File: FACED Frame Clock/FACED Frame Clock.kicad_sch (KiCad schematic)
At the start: 49 parts, among them J1 Jack-DC, U1 LT1711xMS8, U2 LT1711xMS8, U3 LT1711xMS8, U4 LT1711xMS8, U5 Itsy_Bitsy_32u4, U6 SN74AC08PWR, U7 SN74AC08PWR

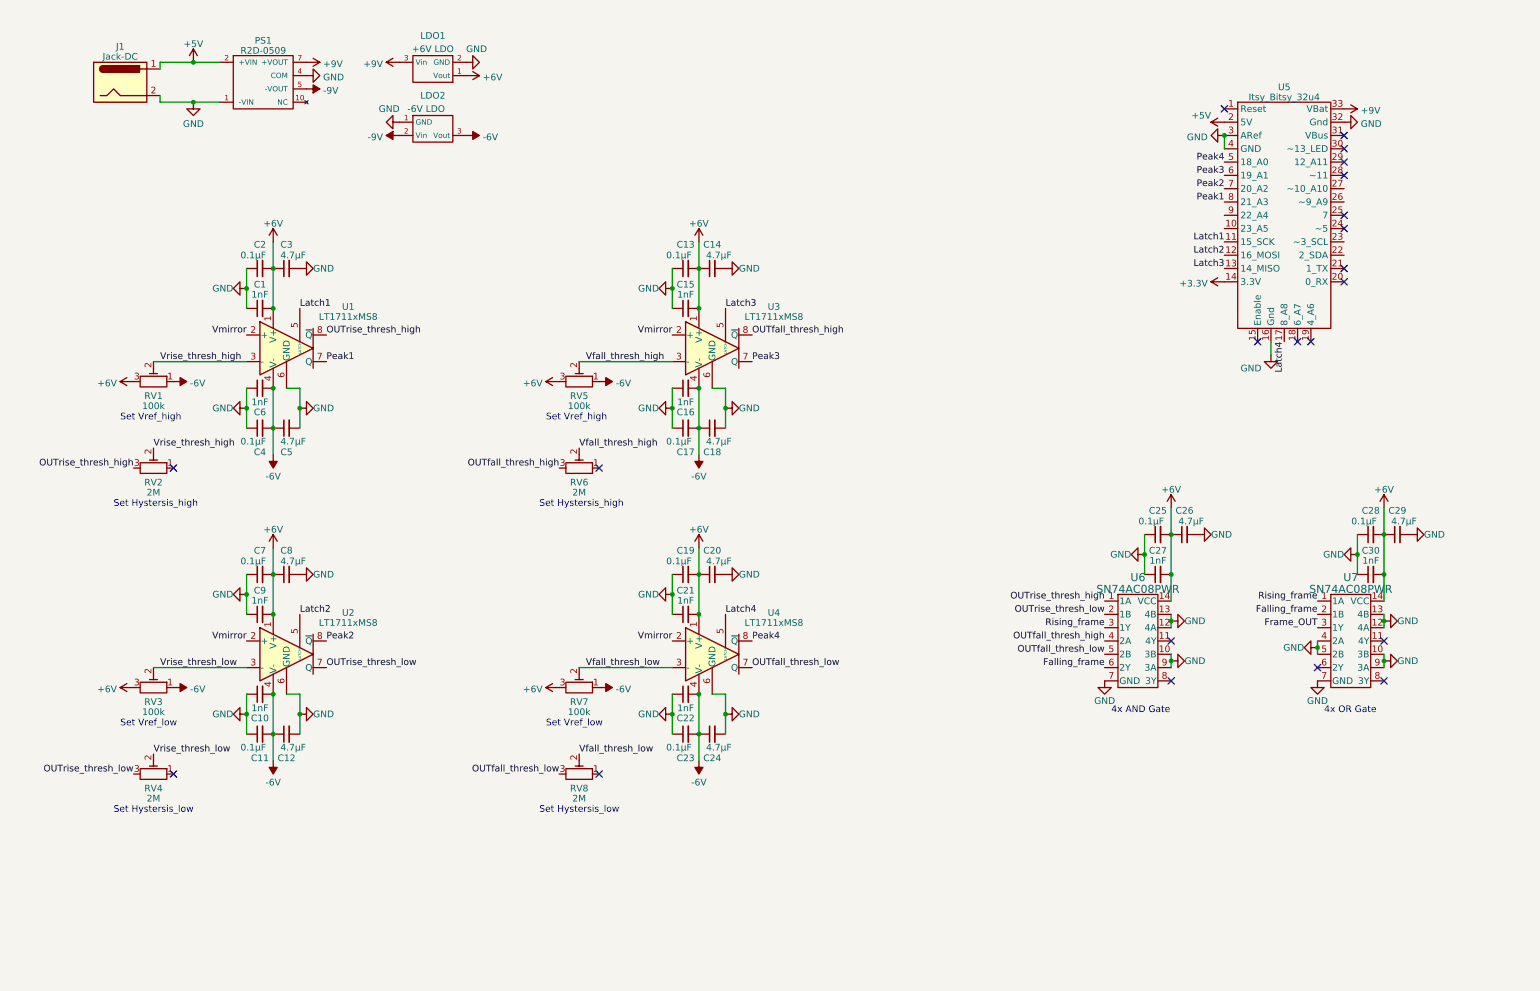
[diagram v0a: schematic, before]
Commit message: Label schematic
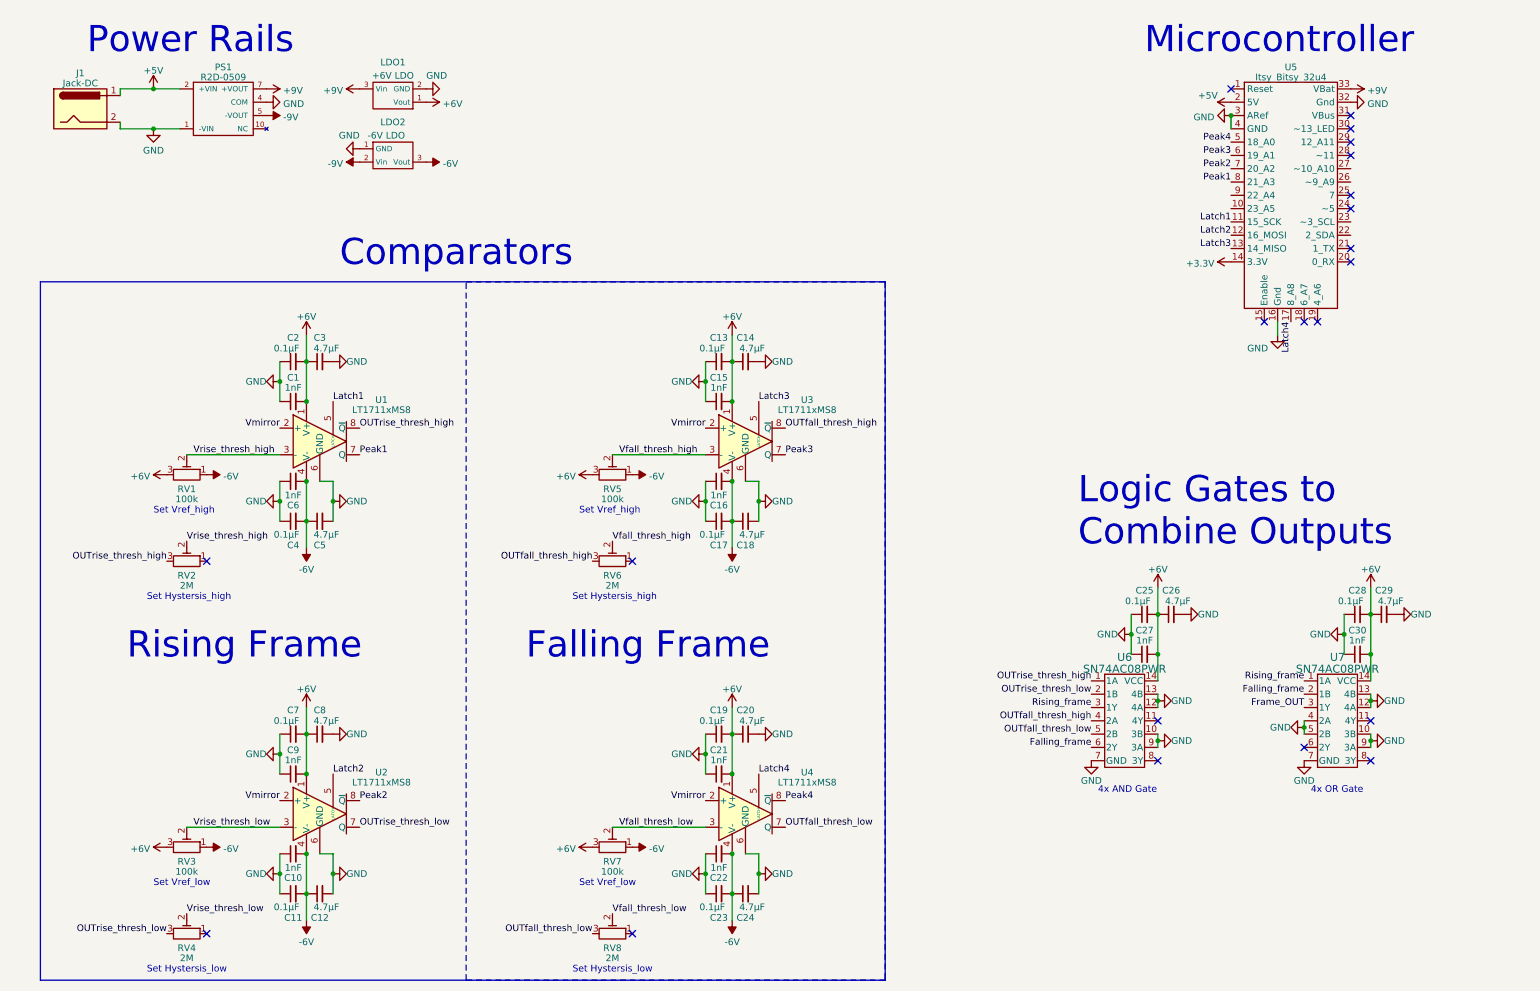
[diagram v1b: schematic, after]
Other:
- note added: "Comparators"
- note added: "Falling Frame"
- note added: "Logic Gates to Combine Outputs"
- note added: "Microcontroller"
- note added: "Power Rails"
- note added: "Rising Frame"
- moved on the sheet: C1, C10, C11, C12, C13, C14, C15, C16, C17, C18, C19, C2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

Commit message: Working draft of simplified version
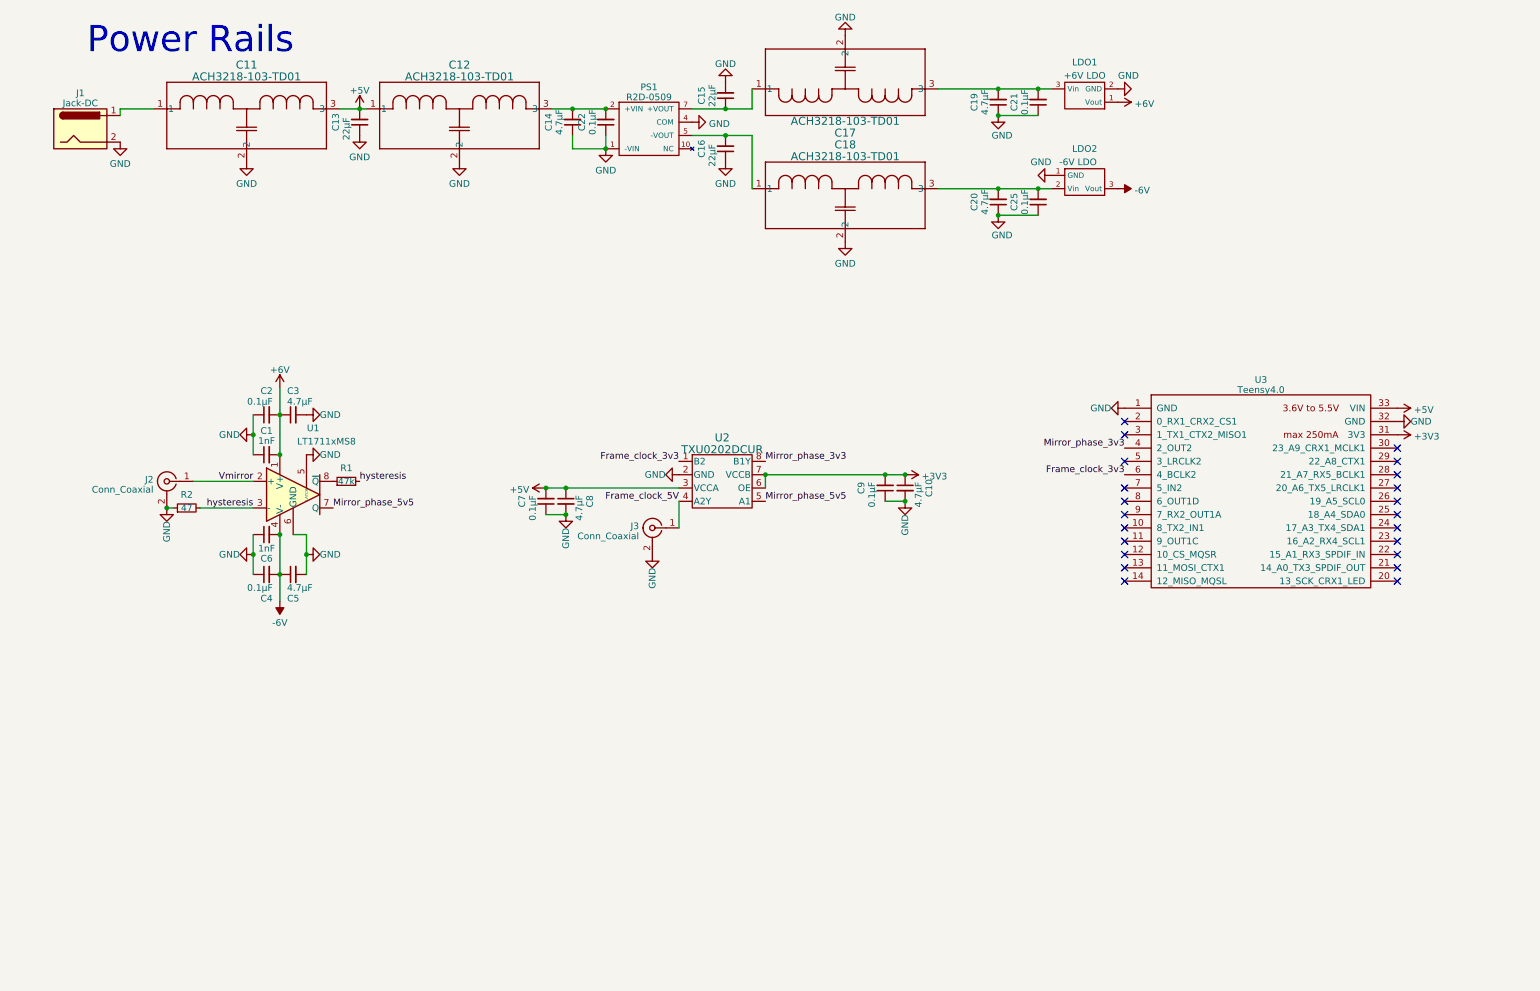
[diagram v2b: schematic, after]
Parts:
- removed C11, C17, C23, C28: 0.1µF, Capacitor_SMD:C_0603_1608Metric, symbol Device:C_Small
- removed C12, C18, C24, C26, C29: 4.7µF, Capacitor_SMD:C_0603_1608Metric, symbol Device:C_Small
- removed C27, C30: 1nF, Capacitor_SMD:C_0603_1608Metric, symbol Device:C_Small
- removed RV1, RV3, RV5, RV7: 100k, Custom footprints:TRIM_TS63Y104KT20, symbol Device:R_Potentiometer_Trim
- removed RV2, RV4, RV6, RV8: 2M, Custom footprints:TRIM_TS63Y104KT20, symbol Device:R_Potentiometer_Trim
- removed U2, U3, U4: LT1711xMS8, Package_SO:MSOP-8_3x3mm_P0.65mm, symbol Comparator:LT1711xMS8
- removed U5: Itsy_Bitsy_32u4, Custom footprints:Itsy Bitsy 32u4, symbol custom:Itsy_Bitsy_32u4
- removed U6, U7: SN74AC08PWR, PW14, symbol Custom:SN74AC08PWR
- added C11: ACH3218-103-TD01, Custom footprints:CAP_TDK_ACH3218_TDK, symbol Custom:ACH3218-103-TD01
- added C12, C17, C18: ACH3218-103-TD01, CAP_TDK_ACH3218_TDK, symbol Custom:ACH3218-103-TD01
- added J2, J3: Conn_Coaxial, Custom footprints:LINX_CONSMA001-C-G, symbol Connector:Conn_Coaxial
- added R1: 47k, Resistor_SMD:R_0805_2012Metric, symbol Device:R_Small
- added R2: 47, Resistor_SMD:R_0603_1608Metric, symbol Device:R_Small
- added U2: TXU0202DCUR, Custom footprints:TXU0202DCUR, symbol Custom:TXU0202DCUR
- added U3: Teensy4.0, Custom footprints:Teensy40-with headers, symbol teensy:Teensy4.0-header_only
- C10: value 1nF -> 4.7µF; Manufacturer TDK Corporation -> Samsung Electro-Mechanics; Part CGA3E2X7R2A102K080AA -> CL10A475KP8NNNC
- C13: value 0.1µF -> 22µF; footprint Capacitor_SMD:C_0603_1608Metric -> Capacitor_SMD:C_0805_2012Metric; Manufacturer TDK Corporation -> Samsung Electro-Mechanics; Part C1608X7R1H104K080AA -> CL21A226MAYNNNE
- C15, C16: value 1nF -> 22µF; footprint Capacitor_SMD:C_0603_1608Metric -> Capacitor_SMD:C_0805_2012Metric; Manufacturer TDK Corporation -> Samsung Electro-Mechanics; Part CGA3E2X7R2A102K080AA -> CL21A226MAYNNNE
- C19: value 0.1µF -> 4.7µF; Manufacturer TDK Corporation -> Samsung Electro-Mechanics; Part C1608X7R1H104K080AA -> CL10A475KP8NNNC
- C21, C22, C9: value 1nF -> 0.1µF; Part CGA3E2X7R2A102K080AA -> C1608X7R1H104K080AA
- PS1: footprint R2D-0509:CONV_R2D-0509 -> Custom footprints:CONV_R2D-0509; MANUFACTURER RECOM -> (none); MAXIMUM_PACKAGE_HEIGHT 9.0mm -> (none); Manufacturer (none) -> Recom Power; PARTREV 0 -> (none); Part (none) -> R2D-0509; STANDARD Manufacturer Recommendations -> (none)
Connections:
- net Latch1 is gone; now on net GND: U1.5 (LATCH)
- net +5V: now also C13.2, C7.2, C8.1, C11.3, C12.1, U2.3 (VCCA), U3.33 (VIN); no longer J1.1, PS1.2 (+VIN)
- net +6V: no longer C13.2, C14.1, C15.2, C19.2, C20.1, C21.2, C25.2, C7.2, C8.1, C9.2
- net -6V: no longer C10.2, C16.2, C22.2
- net GND: now also C10.2, C14.1, C15.2, C20.1, C11.2, C12.2, C17.2, C18.2, J2.2 (Ext), J3.2 (Ext), R2.1, U2.2 (GND), U3.1 (GND), U3.32 (GND); no longer C10.1, C14.2, C15.1, C20.2
- net Vmirror: now also J2.1 (In)
- net +9V: no longer names the net of LDO1.3 (Vin)
- net +9V: now also C19.2, C21.2, C17.3; no longer PS1.7 (+VOUT)
- net -9V: no longer names the net of LDO2.2 (Vin)
- net -9V: now also C20.2, C25.2, C18.3; no longer PS1.5 (-VOUT)
- net OUTrise_thresh_high: no longer names the net of U1.8 (~{Q})
- net OUTrise_thresh_high: now also R1.1
- net Peak1 renamed Mirror_phase_5v5
- net Mirror_phase_5v5: now also U2.5 (A1)
- net Vrise_thresh_high renamed hysteresis
- net hysteresis: now also R1.2, R2.2
- new net: C12.3, C14.2, C22.2, PS1.2 (+VIN)
- new net: C11.1, J1.1
- new net: C15.1, C17.1, PS1.7 (+VOUT)
- new net: C16.2, C18.1, PS1.5 (-VOUT)
- new net +3V3: C10.1, C9.2, U2.6 (OE), U2.7 (VCCB), U3.31 (3V3)
- new net Frame_clock_3v3: U2.1 (B2), U3.6 (4_BCLK2)
- new net Frame_clock_5V: J3.1 (In), U2.4 (A2Y)
- new net Mirror_phase_3v3: U2.8 (B1Y), U3.4 (2_OUT2)
- no-connect marks 21 -> 22
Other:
- note removed: "4x AND Gate"
- note removed: "4x OR Gate"
- note removed: "Comparators"
- note removed: "Falling Frame"
- note removed: "Logic Gates to Combine Outputs"
- note removed: "Microcontroller"
- note removed: "Rising Frame"
- note removed: "Set Hystersis_high"
- note removed: "Set Hystersis_low"
- note removed: "Set Vref_high"
- note removed: "Set Vref_low"
- moved on the sheet: C1, C2, C3, C4, C5, C6, J1, LDO1, LDO2, PS1, U1
